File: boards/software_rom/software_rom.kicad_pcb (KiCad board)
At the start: 2 copper layers, 51.4 x 41.9 mm, 19 parts, among them J1 Conn_02x10_Top_Bottom, J2 uart_conn, J3 ICSP, SW1 SW_Push, U1 ATmega328P-P, Y1 16MHz

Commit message: change values according to actual parts
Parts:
- R1: value 5k -> 3.9k
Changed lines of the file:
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@@
       (effects (font (size 1 1) (thickness 0.15)) (justify mirror))
     )
-    (fp_text value "5k" (at 0 -1.65) (layer "B.Fab")
+    (fp_text value "3.9k" (at 0 -1.65) (layer "B.Fab")
       (effects (font (size 1 1) (thickness 0.15)) (justify mirror))
     )

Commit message: adjust for creating gerver files
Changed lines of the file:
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@@
   (setup
     (pad_to_mask_clearance 0)
+    (aux_axis_origin 144.145 74.295)
     (pcbplotparams
-      (layerselection 0x00010fc_ffffffff)
+      (layerselection 0x00010f0_ffffffff)
       (disableapertmacros false)
       (usegerberextensions false)
@@
       (viasonmask false)
       (mode 1)
-      (useauxorigin false)
+      (useauxorigin true)
       (hpglpennumber 1)
       (hpglpenspeed 20)
@@
       (outputformat 1)
       (mirror false)
-      (drillshape 1)
+      (drillshape 0)
       (scaleselection 1)
-      (outputdirectory "")
+      (outputdirectory "../../../release/todo_tag_here/work/software_rom/")
     )
   )
@@
     (fp_line (start -0.7 -0.6) (end -1 -0.3) (layer "F.Fab") (width 0.1))
     (fp_line (start 1 -0.6) (end -0.7 -0.6) (layer "F.Fab") (width 0.1))
-    (pad "1" smd roundrect (at -1.025 0 180) (size 1.15 1.4) (layers "F.Cu" "F.Paste" "F.Mask") (roundrect_rratio 0.217391)
+    (pad "1" smd roundrect (at -1.025 0 180) (size 1.15 1.4) (layers "F.Cu" "F.Paste" "F.Mask") (roundrect_rratio 0.2173913043)
       (net 1 "GND") (pinfunction "K") (pintype "passive"))
-    (pad "2" smd roundrect (at 1.025 0 180) (size 1.15 1.4) (layers "F.Cu" "F.Paste" "F.Mask") (roundrect_rratio 0.217391)
+    (pad "2" smd roundrect (at 1.025 0 180) (size 1.15 1.4) (layers "F.Cu" "F.Paste" "F.Mask") (roundrect_rratio 0.2173913043)
       (net 8 "Net-(D1-Pad2)") (pinfunction "A") (pintype "passive"))
     (model "${KICAD6_3DMODEL_DIR}/LED_SMD.3dshapes/LED_0805_2012Metric.wrl"
@@
     (fp_line (start -1 -0.625) (end -1 0.625) (layer "B.Fab") (width 0.1))
     (fp_line (start -1 0.625) (end 1 0.625) (layer "B.Fab") (width 0.1))
-    (pad "1" smd roundrect (at -1 0 180) (size 1.2 1.4) (layers "B.Cu" "B.Paste" "B.Mask") (roundrect_rratio 0.208333)
+    (pad "1" smd roundrect (at -1 0 180) (size 1.2 1.4) (layers "B.Cu" "B.Paste" "B.Mask") (roundrect_rratio 0.2083333333)
       (net 29 "/led") (pintype "passive"))
-    (pad "2" smd roundrect (at 1 0 180) (size 1.2 1.4) (layers "B.Cu" "B.Paste" "B.Mask") (roundrect_rratio 0.208333)
+    (pad "2" smd roundrect (at 1 0 180) (size 1.2 1.4) (layers "B.Cu" "B.Paste" "B.Mask") (roundrect_rratio 0.2083333333)
       (net 8 "Net-(D1-Pad2)") (pintype "passive"))
     (model "${KICAD6_3DMODEL_DIR}/Resistor_SMD.3dshapes/R_0805_2012Metric.wrl"
@@
     (fp_line (start 1 -0.625) (end -1 -0.625) (layer "B.Fab") (width 0.1))
     (fp_line (start -1 0.625) (end 1 0.625) (layer "B.Fab") (width 0.1))
-    (pad "1" smd roundrect (at -1 0 180) (size 1.2 1.4) (layers "B.Cu" "B.Paste" "B.Mask") (roundrect_rratio 0.208333)
+    (pad "1" smd roundrect (at -1 0 180) (size 1.2 1.4) (layers "B.Cu" "B.Paste" "B.Mask") (roundrect_rratio 0.2083333333)
       (net 2 "VCC") (pintype "passive"))
-    (pad "2" smd roundrect (at 1 0 180) (size 1.2 1.4) (layers "B.Cu" "B.Paste" "B.Mask") (roundrect_rratio 0.208333)
+    (pad "2" smd roundrect (at 1 0 180) (size 1.2 1.4) (layers "B.Cu" "B.Paste" "B.Mask") (roundrect_rratio 0.2083333333)
       (net 30 "Net-(R4-Pad2)") (pintype "passive"))
     (model "${KICAD6_3DMODEL_DIR}/Resistor_SMD.3dshapes/R_0805_2012Metric.wrl"
@@
     (fp_line (start 1 0.625) (end 1 -0.625) (layer "B.Fab") (width 0.1))
     (fp_line (start 1 -0.625) (end -1 -0.625) (layer "B.Fab") (width 0.1))
-    (pad "1" smd roundrect (at -1.0375 0 180) (size 1.175 1.45) (layers "B.Cu" "B.Paste" "B.Mask") (roundrect_rratio 0.212766)
+    (pad "1" smd roundrect (at -1.0375 0 180) (size 1.175 1.45) (layers "B.Cu" "B.Paste" "B.Mask") (roundrect_rratio 0.2127659574)
       (net 6 "/xtal1") (pintype "passive"))
-    (pad "2" smd roundrect (at 1.0375 0 180) (size 1.175 1.45) (layers "B.Cu" "B.Paste" "B.Mask") (roundrect_rratio 0.212766)
+    (pad "2" smd roundrect (at 1.0375 0 180) (size 1.175 1.45) (layers "B.Cu" "B.Paste" "B.Mask") (roundrect_rratio 0.2127659574)
       (net 1 "GND") (pintype "passive"))
     (model "${KICAD6_3DMODEL_DIR}/Capacitor_SMD.3dshapes/C_0805_2012Metric.wrl"
@@
     (fp_line (start -1 -0.625) (end -1 0.625) (layer "B.Fab") (width 0.1))
     (fp_line (start 1 -0.625) (end -1 -0.625) (layer "B.Fab") (width 0.1))
-    (pad "1" smd roundrect (at -1.0375 0) (size 1.175 1.45) (layers "B.Cu" "B.Paste" "B.Mask") (roundrect_rratio 0.212766)
+    (pad "1" smd roundrect (at -1.0375 0) (size 1.175 1.45) (layers "B.Cu" "B.Paste" "B.Mask") (roundrect_rratio 0.2127659574)
       (net 4 "Net-(C3-Pad1)") (pintype "passive"))
-    (pad "2" smd roundrect (at 1.0375 0) (size 1.175 1.45) (layers "B.Cu" "B.Paste" "B.Mask") (roundrect_rratio 0.212766)
+    (pad "2" smd roundrect (at 1.0375 0) (size 1.175 1.45) (layers "B.Cu" "B.Paste" "B.Mask") (roundrect_rratio 0.2127659574)
       (net 5 "/reset") (pintype "passive"))
     (model "${KICAD6_3DMODEL_DIR}/Capacitor_SMD.3dshapes/C_0805_2012Metric.wrl"
@@
     (fp_line (start -1 0.625) (end 1 0.625) (layer "B.Fab") (width 0.1))
     (fp_line (start -1 -0.625) (end -1 0.625) (layer "B.Fab") (width 0.1))
-    (pad "1" smd roundrect (at -1.0375 0 180) (size 1.175 1.45) (layers "B.Cu" "B.Paste" "B.Mask") (roundrect_rratio 0.212766)
+    (pad "1" smd roundrect (at -1.0375 0 180) (size 1.175 1.45) (layers "B.Cu" "B.Paste" "B.Mask") (roundrect_rratio 0.2127659574)
       (net 7 "/xtal2") (pintype "passive"))
-    (pad "2" smd roundrect (at 1.0375 0 180) (size 1.175 1.45) (layers "B.Cu" "B.Paste" "B.Mask") (roundrect_rratio 0.212766)
+    (pad "2" smd roundrect (at 1.0375 0 180) (size 1.175 1.45) (layers "B.Cu" "B.Paste" "B.Mask") (roundrect_rratio 0.2127659574)
       (net 1 "GND") (pintype "passive"))
     (model "${KICAD6_3DMODEL_DIR}/Capacitor_SMD.3dshapes/C_0805_2012Metric.wrl"
@@
     (fp_line (start 1 0.625) (end 1 -0.625) (layer "B.Fab") (width 0.1))
     (fp_line (start -1 -0.625) (end -1 0.625) (layer "B.Fab") (width 0.1))
-    (pad "1" smd roundrect (at -1 0 180) (size 1.2 1.4) (layers "B.Cu" "B.Paste" "B.Mask") (roundrect_rratio 0.208333)
+    (pad "1" smd roundrect (at -1 0 180) (size 1.2 1.4) (layers "B.Cu" "B.Paste" "B.Mask") (roundrect_rratio 0.2083333333)
       (net 25 "/gpio") (pintype "passive"))
-    (pad "2" smd roundrect (at 1 0 180) (size 1.2 1.4) (layers "B.Cu" "B.Paste" "B.Mask") (roundrect_rratio 0.208333)
+    (pad "2" smd roundrect (at 1 0 180) (size 1.2 1.4) (layers "B.Cu" "B.Paste" "B.Mask") (roundrect_rratio 0.2083333333)
       (net 30 "Net-(R4-Pad2)") (pintype "passive"))
     (model "${KICAD6_3DMODEL_DIR}/Resistor_SMD.3dshapes/R_0805_2012Metric.wrl"
@@
     (fp_line (start -1 0.625) (end 1 0.625) (layer "B.Fab") (width 0.1))
     (fp_line (start -1 -0.625) (end -1 0.625) (layer "B.Fab") (width 0.1))
-    (pad "1" smd roundrect (at -1.0375 0 270) (size 1.175 1.45) (layers "B.Cu" "B.Paste" "B.Mask") (roundrect_rratio 0.212766)
+    (pad "1" smd roundrect (at -1.0375 0 270) (size 1.175 1.45) (layers "B.Cu" "B.Paste" "B.Mask") (roundrect_rratio 0.2127659574)
       (net 1 "GND") (pintype "passive"))
-    (pad "2" smd roundrect (at 1.0375 0 270) (size 1.175 1.45) (layers "B.Cu" "B.Paste" "B.Mask") (roundrect_rratio 0.212766)
+    (pad "2" smd roundrect (at 1.0375 0 270) (size 1.175 1.45) (layers "B.Cu" "B.Paste" "B.Mask") (roundrect_rratio 0.2127659574)
       (net 2 "VCC") (pintype "passive"))
     (model "${KICAD6_3DMODEL_DIR}/Capacitor_SMD.3dshapes/C_0805_2012Metric.wrl"
@@
     (fp_line (start -1 -0.625) (end -1 0.625) (layer "B.Fab") (width 0.1))
     (fp_line (start -1 0.625) (end 1 0.625) (layer "B.Fab") (width 0.1))
-    (pad "1" smd roundrect (at -1 0) (size 1.2 1.4) (layers "B.Cu" "B.Paste" "B.Mask") (roundrect_rratio 0.208333)
+    (pad "1" smd roundrect (at -1 0) (size 1.2 1.4) (layers "B.Cu" "B.Paste" "B.Mask") (roundrect_rratio 0.2083333333)
       (net 4 "Net-(C3-Pad1)") (pintype "passive"))
-    (pad "2" smd roundrect (at 1 0) (size 1.2 1.4) (layers "B.Cu" "B.Paste" "B.Mask") (roundrect_rratio 0.208333)
+    (pad "2" smd roundrect (at 1 0) (size 1.2 1.4) (layers "B.Cu" "B.Paste" "B.Mask") (roundrect_rratio 0.2083333333)
       (net 1 "GND") (pintype "passive"))
     (model "${KICAD6_3DMODEL_DIR}/Resistor_SMD.3dshapes/R_0805_2012Metric.wrl"
@@
     (fp_line (start -1 0.625) (end 1 0.625) (layer "B.Fab") (width 0.1))
     (fp_line (start 1 -0.625) (end -1 -0.625) (layer "B.Fab") (width 0.1))
-    (pad "1" smd roundrect (at -1.0375 0 270) (size 1.175 1.45) (layers "B.Cu" "B.Paste" "B.Mask") (roundrect_rratio 0.212766)
+    (pad "1" smd roundrect (at -1.0375 0 270) (size 1.175 1.45) (layers "B.Cu" "B.Paste" "B.Mask") (roundrect_rratio 0.2127659574)
       (net 3 "Net-(C2-Pad1)") (pintype "passive"))
-    (pad "2" smd roundrect (at 1.0375 0 270) (size 1.175 1.45) (layers "B.Cu" "B.Paste" "B.Mask") (roundrect_rratio 0.212766)
+    (pad "2" smd roundrect (at 1.0375 0 270) (size 1.175 1.45) (layers "B.Cu" "B.Paste" "B.Mask") (roundrect_rratio 0.2127659574)
       (net 1 "GND") (pintype "passive"))
     (model "${KICAD6_3DMODEL_DIR}/Capacitor_SMD.3dshapes/C_0805_2012Metric.wrl"
@@
     (fp_line (start -1 0.625) (end 1 0.625) (layer "B.Fab") (width 0.1))
     (fp_line (start -1 -0.625) (end -1 0.625) (layer "B.Fab") (width 0.1))
-    (pad "1" smd roundrect (at -1 0 180) (size 1.2 1.4) (layers "B.Cu" "B.Paste" "B.Mask") (roundrect_rratio 0.208333)
+    (pad "1" smd roundrect (at -1 0 180) (size 1.2 1.4) (layers "B.Cu" "B.Paste" "B.Mask") (roundrect_rratio 0.2083333333)
       (net 2 "VCC") (pintype "passive"))
-    (pad "2" smd roundrect (at 1 0 180) (size 1.2 1.4) (layers "B.Cu" "B.Paste" "B.Mask") (roundrect_rratio 0.208333)
+    (pad "2" smd roundrect (at 1 0 180) (size 1.2 1.4) (layers "B.Cu" "B.Paste" "B.Mask") (roundrect_rratio 0.2083333333)
       (net 5 "/reset") (pintype "passive"))
     (model "${KICAD6_3DMODEL_DIR}/Resistor_SMD.3dshapes/R_0805_2012Metric.wrl"

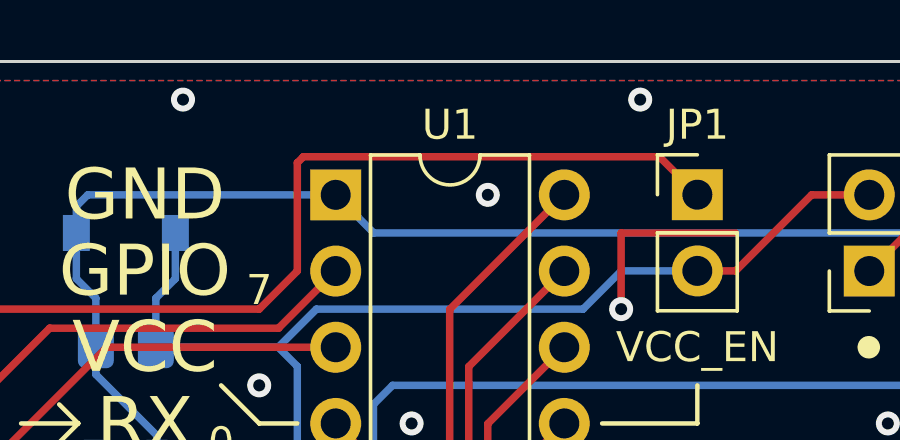
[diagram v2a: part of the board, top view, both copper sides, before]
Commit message: unify libraries
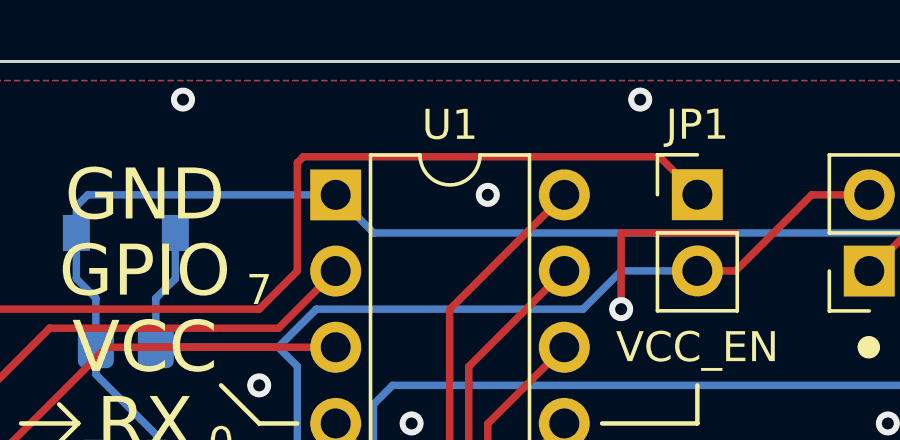
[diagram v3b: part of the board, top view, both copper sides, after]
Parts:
- J1: footprint PrjLibrary_MainBoard:PinHeader_2x10_P2.54mm_Vertical_Top_Bottom -> ModifiedKiCadLibrary:PinHeader_2x10_P2.54mm_Vertical_Top_Bottom
- U1: footprint PrjLibrary_ClockReset:DIP-28_W7.62mm-D1mm -> ModifiedKiCadLibrary:DIP-28_W7.62mm-D1mm
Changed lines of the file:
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@@
     )
   )
-  (footprint "PrjLibrary_ClockReset:DIP-28_W7.62mm-D1mm" (layer "F.Cu")
+  (footprint "ModifiedKiCadLibrary:DIP-28_W7.62mm-D1mm" (layer "F.Cu")
     (at 166.38 78.74)
     (descr "28-lead though-hole mounted DIP package, row spacing 7.62 mm (300 mils) (modified from KiCad 6 library)")
@@
     (property "Sheetname" "")
     (attr through_hole)
-    (fp_text reference "U1" (at 3.81 -2.335) (layer "F.SilkS")
+    (fp_text reference "U1" (at 3.81 -2.33) (layer "F.SilkS")
       (effects (font (size 1 1) (thickness 0.15)))
     )
@@
       (effects (font (size 1 1) (thickness 0.15)))
     )
+    (fp_line (start 6.46 34.35) (end 6.46 -1.33) (layer "F.SilkS") (width 0.12))
     (fp_line (start 1.16 -1.33) (end 1.16 34.35) (layer "F.SilkS") (width 0.12))
     (fp_line (start 6.46 -1.33) (end 4.81 -1.33) (layer "F.SilkS") (width 0.12))
+    (fp_line (start 2.81 -1.33) (end 1.16 -1.33) (layer "F.SilkS") (width 0.12))
     (fp_line (start 1.16 34.35) (end 6.46 34.35) (layer "F.SilkS") (width 0.12))
-    (fp_line (start 2.81 -1.33) (end 1.16 -1.33) (layer "F.SilkS") (width 0.12))
-    (fp_line (start 6.46 34.35) (end 6.46 -1.33) (layer "F.SilkS") (width 0.12))
     (fp_arc (start 4.81 -1.33) (mid 3.81 -0.33) (end 2.81 -1.33) (layer "F.SilkS") (width 0.12))
     (fp_line (start -1.1 34.55) (end 8.7 34.55) (layer "F.CrtYd") (width 0.05))
     (fp_line (start 8.7 -1.55) (end -1.1 -1.55) (layer "F.CrtYd") (width 0.05))
+    (fp_line (start -1.1 -1.55) (end -1.1 34.55) (layer "F.CrtYd") (width 0.05))
     (fp_line (start 8.7 34.55) (end 8.7 -1.55) (layer "F.CrtYd") (width 0.05))
-    (fp_line (start -1.1 -1.55) (end -1.1 34.55) (layer "F.CrtYd") (width 0.05))
+    (fp_line (start 6.985 34.29) (end 0.635 34.29) (layer "F.Fab") (width 0.1))
+    (fp_line (start 6.985 -1.27) (end 6.985 34.29) (layer "F.Fab") (width 0.1))
+    (fp_line (start 0.635 34.29) (end 0.635 -0.27) (layer "F.Fab") (width 0.1))
     (fp_line (start 1.635 -1.27) (end 6.985 -1.27) (layer "F.Fab") (width 0.1))
-    (fp_line (start 0.635 34.29) (end 0.635 -0.27) (layer "F.Fab") (width 0.1))
     (fp_line (start 0.635 -0.27) (end 1.635 -1.27) (layer "F.Fab") (width 0.1))
-    (fp_line (start 6.985 -1.27) (end 6.985 34.29) (layer "F.Fab") (width 0.1))
-    (fp_line (start 6.985 34.29) (end 0.635 34.29) (layer "F.Fab") (width 0.1))
     (pad "1" thru_hole rect (at 0 0) (size 1.7 1.7) (drill 1) (layers *.Cu *.Mask)
       (net 5 "/reset") (pinfunction "~{RESET}/PC6") (pintype "bidirectional"))
@@
     )
   )
-  (footprint "PrjLibrary_MainBoard:PinHeader_2x10_P2.54mm_Vertical_Top_Bottom" (layer "F.Cu")
+  (footprint "ModifiedKiCadLibrary:PinHeader_2x10_P2.54mm_Vertical_Top_Bottom" (layer "F.Cu")
     (at 189.23 88.9)
     (descr "Through hole straight pin header, 2x10, 2.54mm pitch, double rows (modified from KiCad 6 library)")
@@
       (effects (font (size 1 1) (thickness 0.15)))
     )
+    (fp_line (start 3.87 -1.33) (end 3.87 24.19) (layer "F.SilkS") (width 0.12))
+    (fp_line (start -1.33 24.19) (end 3.87 24.19) (layer "F.SilkS") (width 0.12))
+    (fp_line (start 1.27 -1.33) (end 3.87 -1.33) (layer "F.SilkS") (width 0.12))
+    (fp_line (start -1.33 1.27) (end -1.33 24.19) (layer "F.SilkS") (width 0.12))
+    (fp_line (start -1.33 -1.33) (end 0 -1.33) (layer "F.SilkS") (width 0.12))
     (fp_line (start 1.27 1.27) (end 1.27 -1.33) (layer "F.SilkS") (width 0.12))
     (fp_line (start -1.33 1.27) (end 1.27 1.27) (layer "F.SilkS") (width 0.12))
-    (fp_line (start -1.33 24.19) (end 3.87 24.19) (layer "F.SilkS") (width 0.12))
-    (fp_line (start 3.87 -1.33) (end 3.87 24.19) (layer "F.SilkS") (width 0.12))
     (fp_line (start -1.33 0) (end -1.33 -1.33) (layer "F.SilkS") (width 0.12))
-    (fp_line (start 1.27 -1.33) (end 3.87 -1.33) (layer "F.SilkS") (width 0.12))
-    (fp_line (start -1.33 -1.33) (end 0 -1.33) (layer "F.SilkS") (width 0.12))
-    (fp_line (start -1.33 1.27) (end -1.33 24.19) (layer "F.SilkS") (width 0.12))
-    (fp_line (start -1.8 24.65) (end 4.35 24.65) (layer "F.CrtYd") (width 0.05))
     (fp_line (start 4.35 24.65) (end 4.35 -1.8) (layer "F.CrtYd") (width 0.05))
     (fp_line (start 4.35 -1.8) (end -1.8 -1.8) (layer "F.CrtYd") (width 0.05))
     (fp_line (start -1.8 -1.8) (end -1.8 24.65) (layer "F.CrtYd") (width 0.05))
+    (fp_line (start -1.8 24.65) (end 4.35 24.65) (layer "F.CrtYd") (width 0.05))
+    (fp_line (start -1.27 0) (end 0 -1.27) (layer "F.Fab") (width 0.1))
+    (fp_line (start -1.27 24.13) (end -1.27 0) (layer "F.Fab") (width 0.1))
     (fp_line (start 0 -1.27) (end 3.81 -1.27) (layer "F.Fab") (width 0.1))
-    (fp_line (start -1.27 0) (end 0 -1.27) (layer "F.Fab") (width 0.1))
+    (fp_line (start 3.81 -1.27) (end 3.81 24.13) (layer "F.Fab") (width 0.1))
     (fp_line (start 3.81 24.13) (end -1.27 24.13) (layer "F.Fab") (width 0.1))
-    (fp_line (start 3.81 -1.27) (end 3.81 24.13) (layer "F.Fab") (width 0.1))
-    (fp_line (start -1.27 24.13) (end -1.27 0) (layer "F.Fab") (width 0.1))
     (pad "1" thru_hole rect (at 0 0) (size 1.7 1.7) (drill 1) (layers *.Cu *.Mask)
       (net 9 "/addr0") (pinfunction "Pin_1") (pintype "passive"))
